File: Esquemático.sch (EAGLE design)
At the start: 4 parts, among them U1 MPU-6050-1, U2 MPU-6050-1, U3 MPU-6050-1

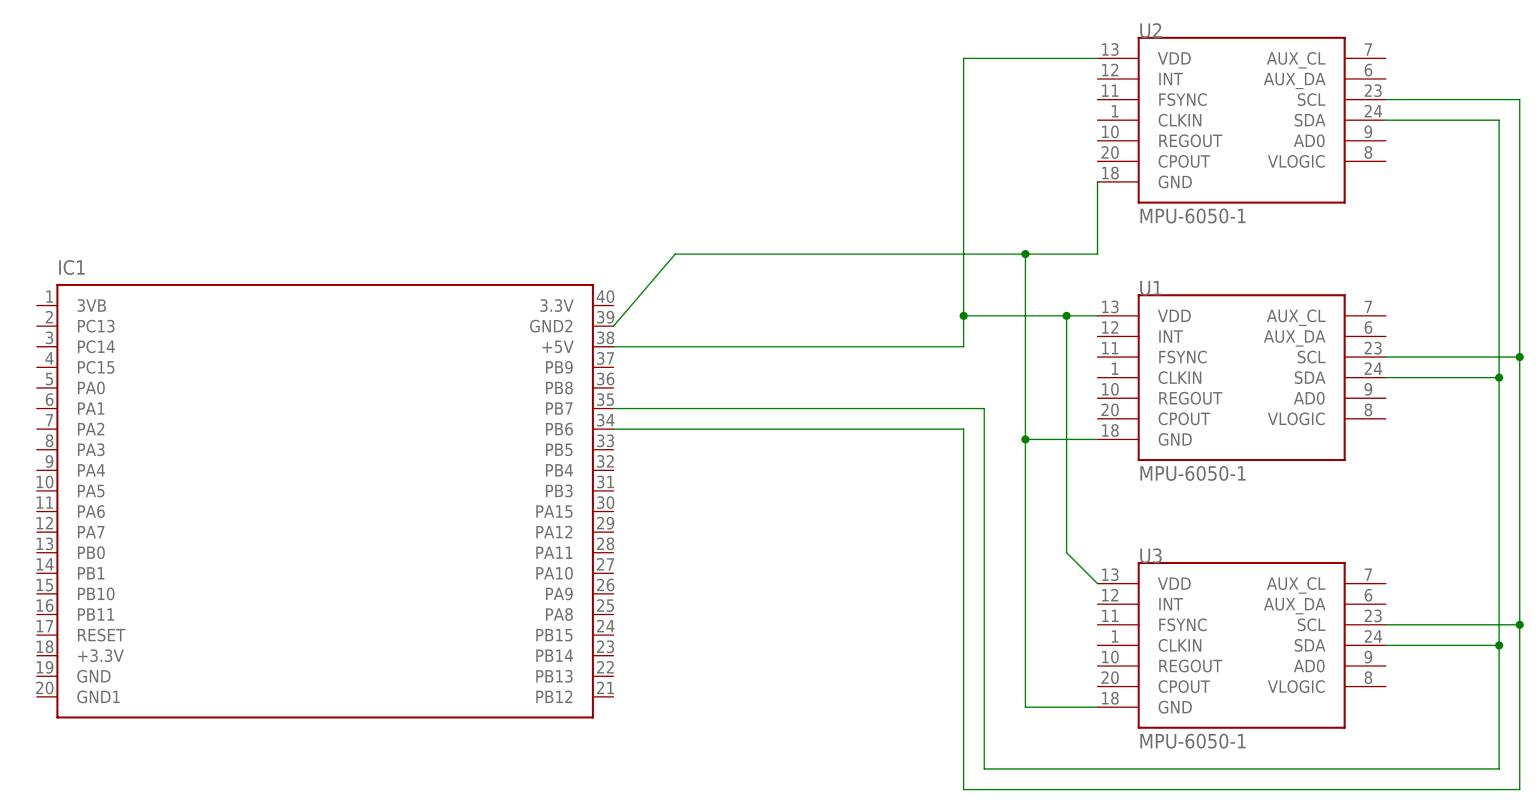
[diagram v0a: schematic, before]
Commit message: Última versão do Esquemático
Presentes tanto:
Esquemático.pdf
Esquemático.png
Esquemático.sch
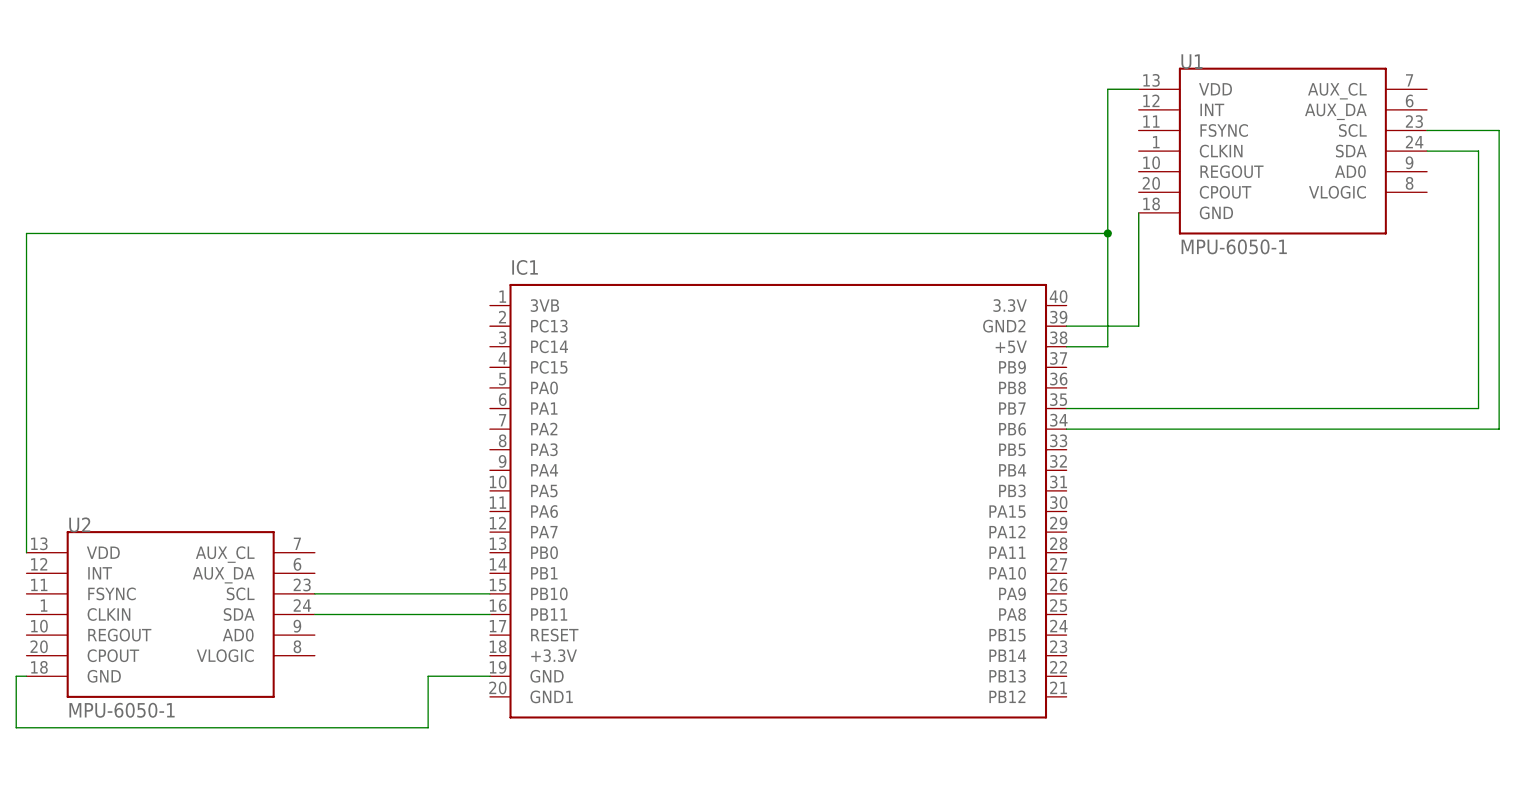
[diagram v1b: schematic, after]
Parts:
- removed U3: MPU-6050-1, Testing:MPU-6050-1
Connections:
- new net N$5: IC1.+5V, U1.VDD, U2.VDD
- new net N$6: IC1.GND2, U1.GND
- new net N$7: IC1.GND, U2.GND
- net N$1: now also IC1.PB10; no longer IC1.PB6, U1.SCL, U3.SCL
- net N$2: no longer U2.SDA, U3.SDA
- net N$3: now also IC1.PB6, U1.SCL; no longer IC1.+5V, U1.VDD, U2.VDD, U3.VDD
- net N$4: now also IC1.PB11, U2.SDA; no longer IC1.GND2, U1.GND, U2.GND, U3.GND
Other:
- moved on the sheet: IC1, U1, U2
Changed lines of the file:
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@@
 <part name="U1" library="Testing" deviceset="MPU-6050" device="-1"/>
 <part name="U2" library="Testing" deviceset="MPU-6050" device="-1"/>
-<part name="U3" library="Testing" deviceset="MPU-6050" device="-1"/>
 </parts>
 <sheets>
@@
 </plain>
 <instances>
-<instance part="IC1" gate="G$1" x="-27.94" y="26.67"/>
-<instance part="U1" gate="G$1" x="85.09" y="43.18"/>
-<instance part="U2" gate="G$1" x="85.09" y="74.93"/>
-<instance part="U3" gate="G$1" x="85.09" y="10.16"/>
+<instance part="IC1" gate="G$1" x="27.94" y="26.67"/>
+<instance part="U1" gate="G$1" x="90.17" y="71.12"/>
+<instance part="U2" gate="G$1" x="-46.99" y="13.97"/>
 </instances>
 <busses>
@@
 <net name="N$1" class="0">
 <segment>
+<pinref part="U2" gate="G$1" pin="SCL"/>
+<pinref part="IC1" gate="G$1" pin="PB10"/>
+<wire x1="-29.21" y1="16.51" x2="-7.62" y2="16.51" width="0.1524" layer="91"/>
+</segment>
+</net>
+<net name="N$3" class="0">
+<segment>
+<pinref part="U1" gate="G$1" pin="SCL"/>
+<wire x1="107.95" y1="73.66" x2="116.84" y2="73.66" width="0.1524" layer="91"/>
 <pinref part="IC1" gate="G$1" pin="PB6"/>
-<wire x1="7.62" y1="36.83" x2="50.8" y2="36.83" width="0.1524" layer="91"/>
-<wire x1="50.8" y1="36.83" x2="50.8" y2="-7.62" width="0.1524" layer="91"/>
-<wire x1="50.8" y1="-7.62" x2="119.38" y2="-7.62" width="0.1524" layer="91"/>
-<wire x1="119.38" y1="-7.62" x2="119.38" y2="12.7" width="0.1524" layer="91"/>
-<pinref part="U2" gate="G$1" pin="SCL"/>
-<wire x1="119.38" y1="12.7" x2="119.38" y2="45.72" width="0.1524" layer="91"/>
-<wire x1="119.38" y1="45.72" x2="119.38" y2="77.47" width="0.1524" layer="91"/>
-<wire x1="119.38" y1="77.47" x2="102.87" y2="77.47" width="0.1524" layer="91"/>
-<pinref part="U1" gate="G$1" pin="SCL"/>
-<wire x1="102.87" y1="45.72" x2="119.38" y2="45.72" width="0.1524" layer="91"/>
-<junction x="119.38" y="45.72"/>
-<pinref part="U3" gate="G$1" pin="SCL"/>
-<wire x1="102.87" y1="12.7" x2="119.38" y2="12.7" width="0.1524" layer="91"/>
-<junction x="119.38" y="12.7"/>
+<wire x1="63.5" y1="36.83" x2="116.84" y2="36.83" width="0.1524" layer="91"/>
+<wire x1="116.84" y1="36.83" x2="116.84" y2="73.66" width="0.1524" layer="91"/>
 </segment>
 </net>
@@
 <segment>
 <pinref part="IC1" gate="G$1" pin="PB7"/>
-<wire x1="7.62" y1="39.37" x2="53.34" y2="39.37" width="0.1524" layer="91"/>
-<wire x1="53.34" y1="39.37" x2="53.34" y2="-5.08" width="0.1524" layer="91"/>
-<wire x1="53.34" y1="-5.08" x2="116.84" y2="-5.08" width="0.1524" layer="91"/>
-<pinref part="U2" gate="G$1" pin="SDA"/>
-<wire x1="116.84" y1="-5.08" x2="116.84" y2="10.16" width="0.1524" layer="91"/>
-<wire x1="116.84" y1="10.16" x2="116.84" y2="43.18" width="0.1524" layer="91"/>
-<wire x1="116.84" y1="43.18" x2="116.84" y2="74.93" width="0.1524" layer="91"/>
-<wire x1="116.84" y1="74.93" x2="102.87" y2="74.93" width="0.1524" layer="91"/>
+<wire x1="63.5" y1="39.37" x2="114.3" y2="39.37" width="0.1524" layer="91"/>
+<wire x1="114.3" y1="39.37" x2="114.3" y2="71.12" width="0.1524" layer="91"/>
 <pinref part="U1" gate="G$1" pin="SDA"/>
-<wire x1="102.87" y1="43.18" x2="116.84" y2="43.18" width="0.1524" layer="91"/>
-<junction x="116.84" y="43.18"/>
-<pinref part="U3" gate="G$1" pin="SDA"/>
-<wire x1="102.87" y1="10.16" x2="116.84" y2="10.16" width="0.1524" layer="91"/>
-<junction x="116.84" y="10.16"/>
-</segment>
-</net>
-<net name="N$3" class="0">
-<segment>
-<pinref part="U2" gate="G$1" pin="VDD"/>
-<wire x1="67.31" y1="82.55" x2="50.8" y2="82.55" width="0.1524" layer="91"/>
-<wire x1="50.8" y1="82.55" x2="50.8" y2="50.8" width="0.1524" layer="91"/>
-<pinref part="IC1" gate="G$1" pin="+5V"/>
-<wire x1="50.8" y1="50.8" x2="50.8" y2="46.99" width="0.1524" layer="91"/>
-<wire x1="7.62" y1="46.99" x2="50.8" y2="46.99" width="0.1524" layer="91"/>
-<pinref part="U1" gate="G$1" pin="VDD"/>
-<wire x1="67.31" y1="50.8" x2="63.5" y2="50.8" width="0.1524" layer="91"/>
-<junction x="50.8" y="50.8"/>
-<pinref part="U3" gate="G$1" pin="VDD"/>
-<wire x1="63.5" y1="50.8" x2="50.8" y2="50.8" width="0.1524" layer="91"/>
-<wire x1="67.31" y1="17.78" x2="63.5" y2="21.59" width="0.1524" layer="91"/>
-<wire x1="63.5" y1="21.59" x2="63.5" y2="50.8" width="0.1524" layer="91"/>
-<junction x="63.5" y="50.8"/>
+<wire x1="114.3" y1="71.12" x2="107.95" y2="71.12" width="0.1524" layer="91"/>
 </segment>
 </net>
 <net name="N$4" class="0">
 <segment>
-<pinref part="U1" gate="G$1" pin="GND"/>
-<wire x1="67.31" y1="35.56" x2="58.42" y2="35.56" width="0.1524" layer="91"/>
-<wire x1="58.42" y1="35.56" x2="58.42" y2="58.42" width="0.1524" layer="91"/>
-<wire x1="58.42" y1="58.42" x2="15.24" y2="58.42" width="0.1524" layer="91"/>
-<pinref part="IC1" gate="G$1" pin="GND2"/>
-<wire x1="15.24" y1="58.42" x2="7.62" y2="49.53" width="0.1524" layer="91"/>
-<pinref part="U2" gate="G$1" pin="GND"/>
-<wire x1="58.42" y1="58.42" x2="67.31" y2="58.42" width="0.1524" layer="91"/>
-<wire x1="67.31" y1="58.42" x2="67.31" y2="67.31" width="0.1524" layer="91"/>
-<junction x="58.42" y="58.42"/>
-<wire x1="58.42" y1="35.56" x2="58.42" y2="2.54" width="0.1524" layer="91"/>
-<junction x="58.42" y="35.56"/>
-<pinref part="U3" gate="G$1" pin="GND"/>
-<wire x1="58.42" y1="2.54" x2="67.31" y2="2.54" width="0.1524" layer="91"/>
+<pinref part="U2" gate="G$1" pin="SDA"/>
+<pinref part="IC1" gate="G$1" pin="PB11"/>
+<wire x1="-29.21" y1="13.97" x2="-7.62" y2="13.97" width="0.1524" layer="91"/>
 </segment>
 </net>
+<net name="N$5" class="0">
+<segment>
+<pinref part="U1" gate="G$1" pin="VDD"/>
+<wire x1="72.39" y1="78.74" x2="68.58" y2="78.74" width="0.1524" layer="91"/>
+<pinref part="IC1" gate="G$1" pin="+5V"/>
+<wire x1="63.5" y1="46.99" x2="68.58" y2="46.99" width="0.1524" layer="91"/>
+<wire x1="68.58" y1="46.99" x2="68.58" y2="60.96" width="0.1524" layer="91"/>
+<pinref part="U2" gate="G$1" pin="VDD"/>
+<wire x1="68.58" y1="60.96" x2="68.58" y2="78.74" width="0.1524" layer="91"/>
+<wire x1="68.58" y1="60.96" x2="-64.77" y2="60.96" width="0.1524" layer="91"/>
+<wire x1="-64.77" y1="60.96" x2="-64.77" y2="21.59" width="0.1524" layer="91"/>
+<junction x="68.58" y="60.96"/>
+</segment>
+</net>
+<net name="N$6" class="0">
+<segment>
+<pinref part="U1" gate="G$1" pin="GND"/>
+<pinref part="IC1" gate="G$1" pin="GND2"/>
+<wire x1="72.39" y1="63.5" x2="72.39" y2="49.53" width="0.1524" layer="91"/>
+<wire x1="72.39" y1="49.53" x2="63.5" y2="49.53" width="0.1524" layer="91"/>
+</segment>
+</net>
+<net name="N$7" class="0">
+<segment>
+<pinref part="IC1" gate="G$1" pin="GND"/>
+<wire x1="-7.62" y1="6.35" x2="-15.24" y2="6.35" width="0.1524" layer="91"/>
+<wire x1="-15.24" y1="6.35" x2="-15.24" y2="0" width="0.1524" layer="91"/>
+<wire x1="-15.24" y1="0" x2="-66.04" y2="0" width="0.1524" layer="91"/>
+<pinref part="U2" gate="G$1" pin="GND"/>
+<wire x1="-66.04" y1="0" x2="-66.04" y2="6.35" width="0.1524" layer="91"/>
+<wire x1="-66.04" y1="6.35" x2="-64.77" y2="6.35" width="0.1524" layer="91"/>
+</segment>
+</net>
